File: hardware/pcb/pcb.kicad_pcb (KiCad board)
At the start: 2 copper layers, 30 x 35 mm, 49 parts, among them CN101 XT30PW-M, U101 RP2040, U102 W25Q128JVP, U103 ICM-42688-P, U104 MIC5219-3.3YM5, U105 MIC5219-3.3YM5, U106 AMS1117-5.0, U107 S4B-XH-SM4-TB-, Y101 12MHz

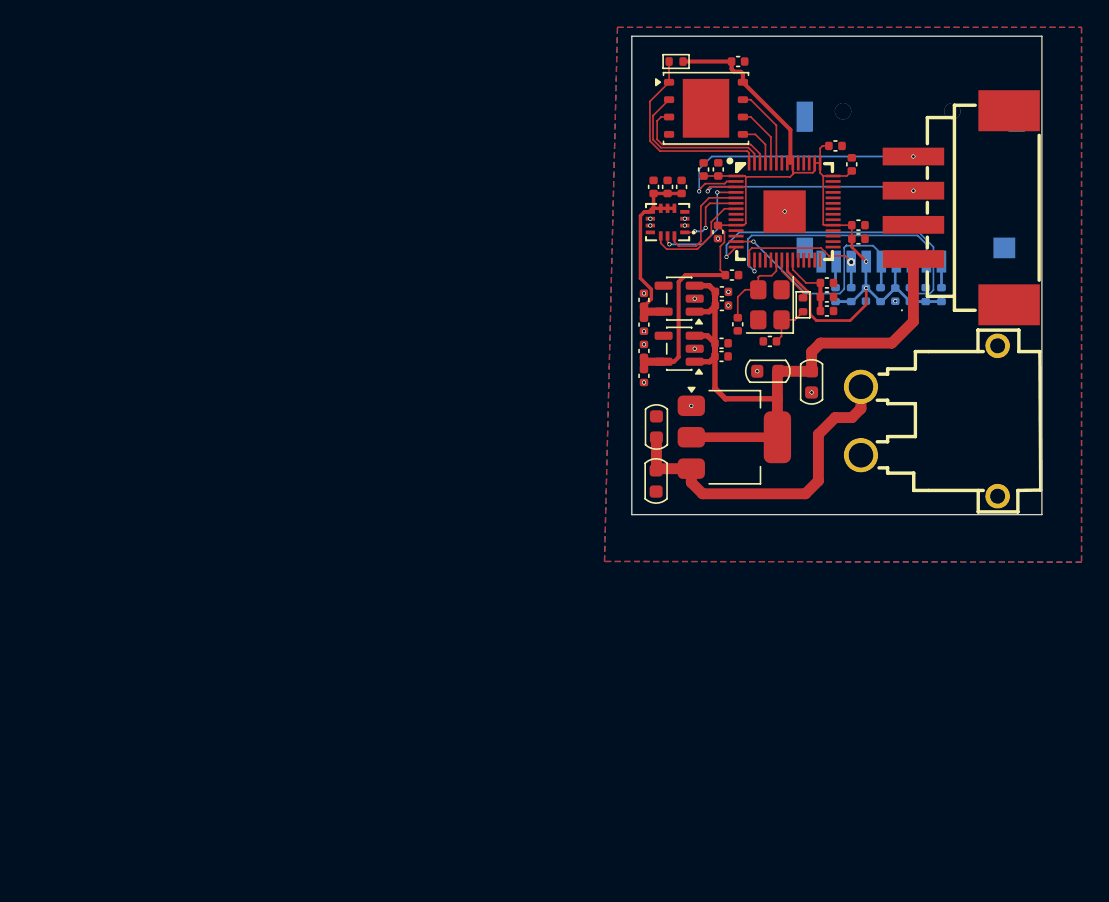
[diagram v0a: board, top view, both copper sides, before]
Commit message: redesign
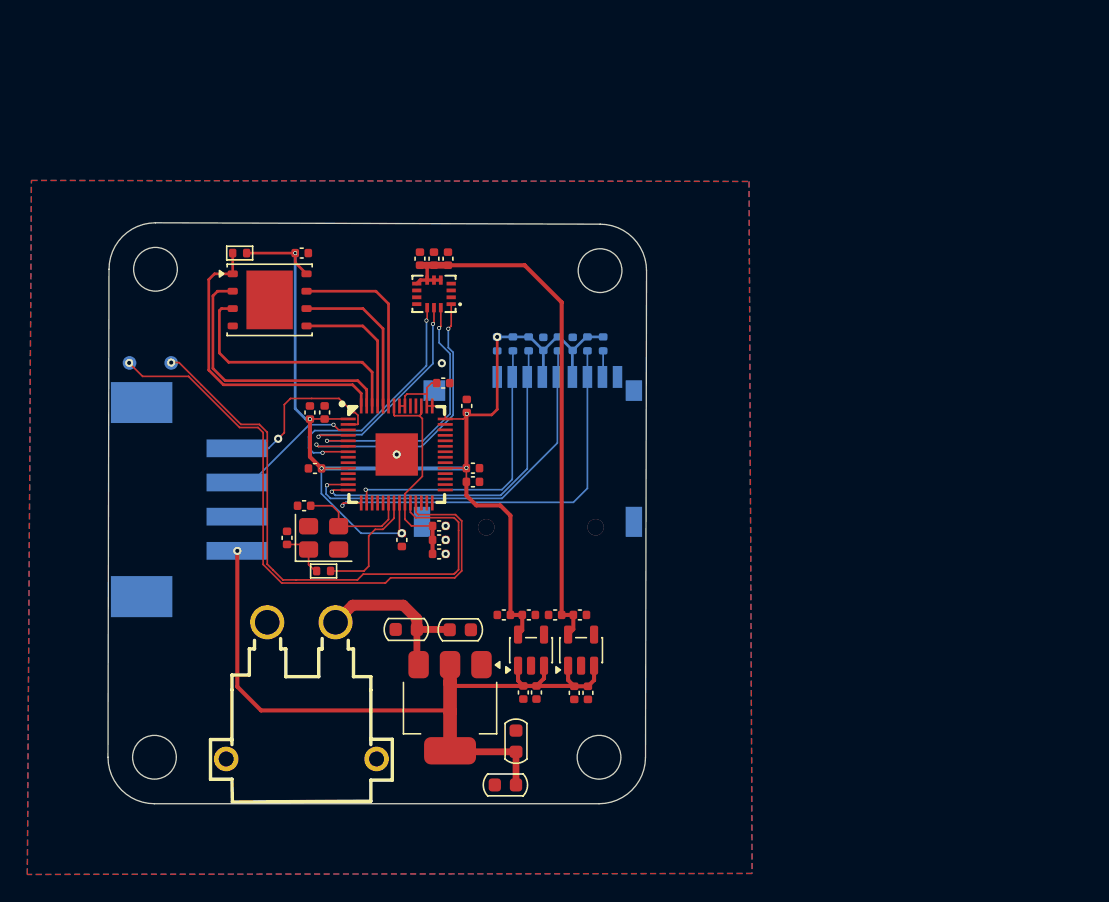
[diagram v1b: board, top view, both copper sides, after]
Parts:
- added H101: MountingHole, MountingHole:MountingHole_3.2mm_M3_DIN965, F.Cu at (87.7, 114.3)
- added H102: MountingHole, MountingHole:MountingHole_3.2mm_M3_DIN965, F.Cu at (120.2, 114.4)
- added H103: MountingHole, MountingHole:MountingHole_3.2mm_M3_DIN965, F.Cu at (87.6, 150.0)
- added H104: MountingHole, MountingHole:MountingHole_3.2mm_M3_DIN965, F.Cu at (120.1, 150.0)
- added TP101: SWCLK, TestPoint:TestPoint_Pad_D1.0mm, B.Cu at (88.8, 121.2)
- added TP102: SWD, TestPoint:TestPoint_Pad_D1.0mm, B.Cu at (85.8, 121.2)
- U107: moved to B.Cu
- moved U107 60.4 mm to (90.1, 131.2)
- moved CN101 50.0 mm to (98.3, 145.1), turned to 0 degrees
- moved R101 40.1 mm to (100.0, 136.4), turned to 0 degrees
- moved C101 38.1 mm to (97.3, 133.9), turned to -90 degrees
- moved C133 37.0 mm to (113.2, 152.0), turned to 180 degrees
- moved Y101 36.8 mm to (100.0, 133.9), turned to 0 degrees
- moved C103 34.9 mm to (98.3, 113.1)
- moved R102 34.9 mm to (93.8, 113.1)
- moved U102 34.9 mm to (96.0, 116.5)
- moved C102 34.4 mm to (98.5, 131.6), turned to 0 degrees
- moved C109 34.2 mm to (99.3, 128.9), turned to 180 degrees
- moved Card101 33.9 mm to (114.9, 127.5), turned to 180 degrees
- moved C114 33.8 mm to (99.0, 124.8)
- moved C113 33.8 mm to (100.0, 124.8)
- moved C108 33.5 mm to (108.7, 122.6)
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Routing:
- net SWD: track 0.00 -> 45.0 mm, vias 0 -> 1
- net SWCLK: track 0.00 -> 41.5 mm, vias 0 -> 1
- net VCC_3V3_GYRO: track 15.5 -> 39.8 mm
- net D0: track 10.6 -> 30.0 mm
- net G_MISO: track 5.51 -> 21.7 mm
- net VCC_3V3: track 83.7 -> 99.9 mm, vias 2 -> 7
- net VBAT: track 25.0 -> 12.7 mm
- net G_MOSI: track 8.04 -> 19.5 mm, vias 0 -> 2
- net G_CS: track 8.01 -> 18.9 mm, vias 0 -> 2
- net VCC_1V1: track 5.17 -> 15.8 mm
- net CLK: track 18.2 -> 27.7 mm
- net G_CLK: track 8.70 -> 16.9 mm
- net 5V: track 48.6 -> 56.8 mm, vias 0 -> 1
- net CS: track 14.8 -> 22.8 mm
- net DO: track 12.0 -> 20.0 mm
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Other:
- board size 30 x 35 mm -> 39.4 x 42.5 mm
